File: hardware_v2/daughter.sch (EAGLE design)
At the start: 25 parts, among them K1 PIN20X2, U1 EEPROM24, U2 MCP2551-I/SN, U4 TPS27081A, X1 MABC48B2

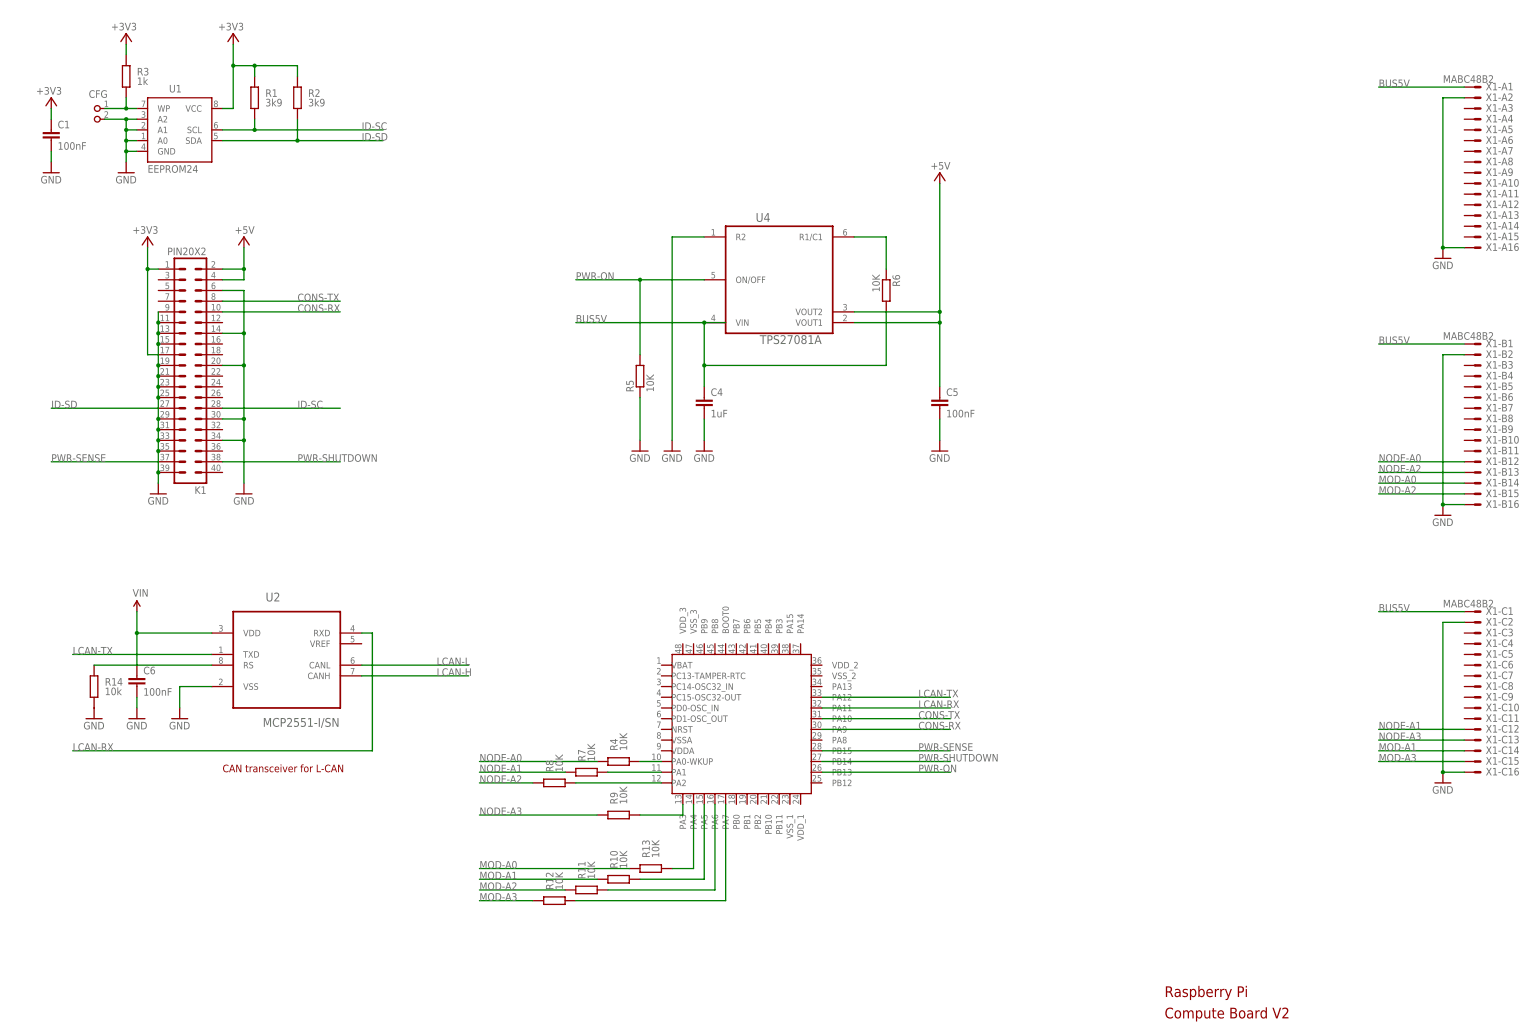
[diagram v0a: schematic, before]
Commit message: hardware_v2: build in STM32
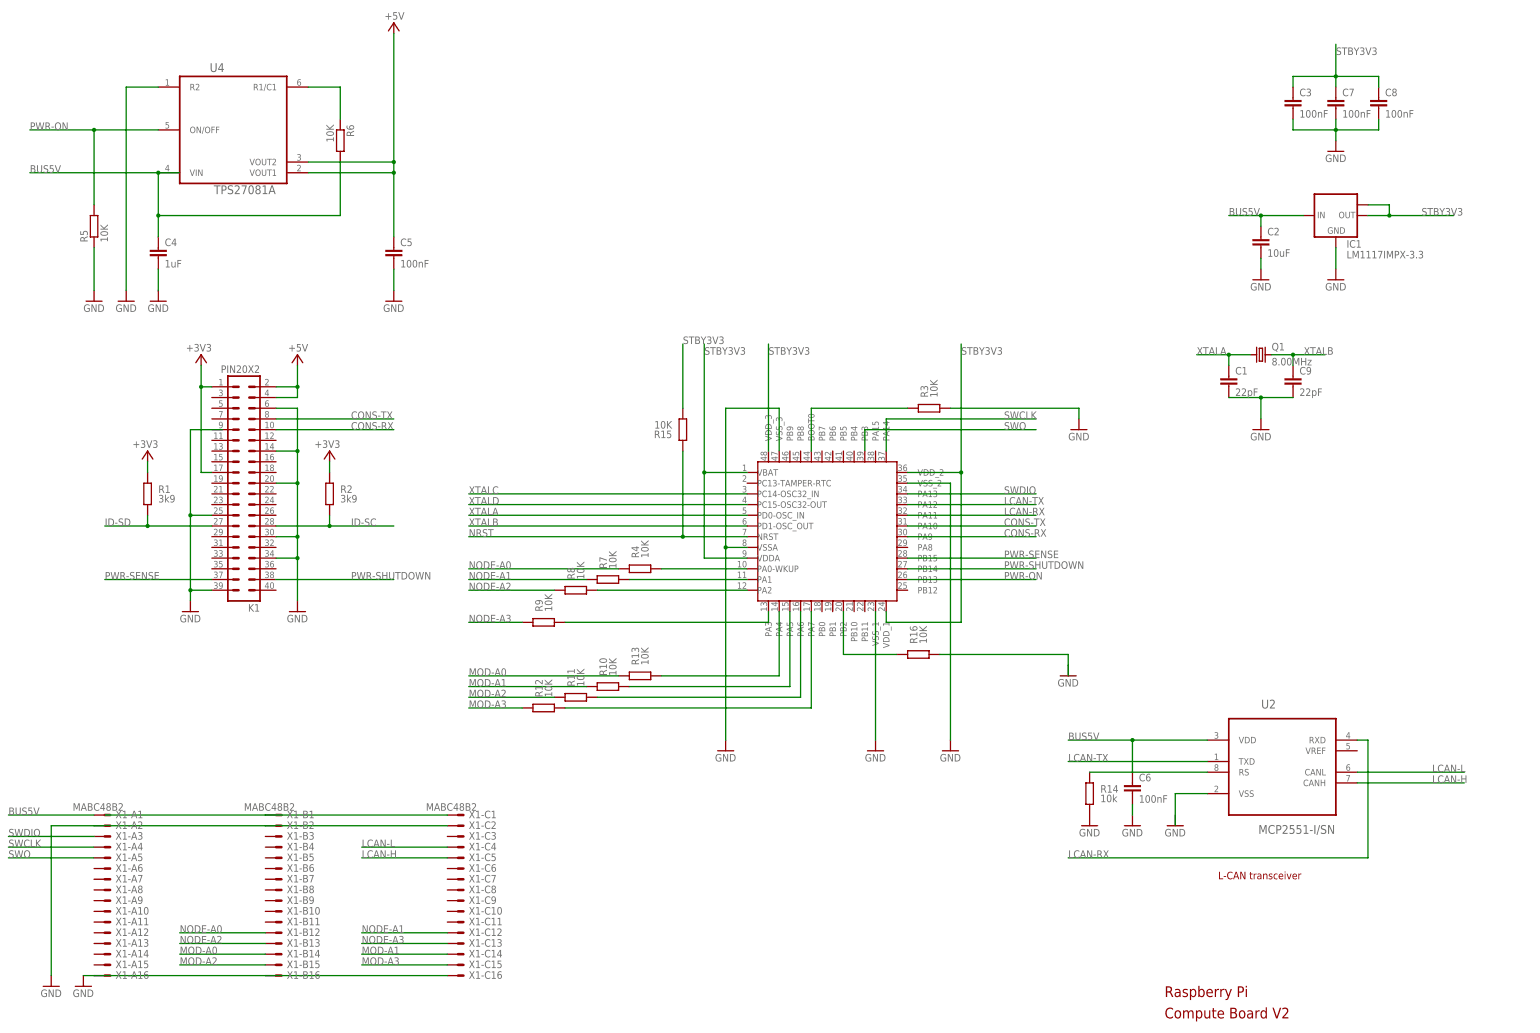
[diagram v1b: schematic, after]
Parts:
- removed CFG: (no value), FLYFISH:PIN2_100
- removed U1: EEPROM24, FLYFISH:EEPROM24
- added C2: 10uF, resistor:C-EUC0805K
- added C3, C7, C8: 100nF, resistor:C-EUC0805K
- added C9: 22pF, resistor:C-EUC1206
- added IC1: LM1117IMPX-3.3, lm1117:LM1117IMPX-3.3
- added Q1: 8.00MHz, crystal:CRYSTALSM49
- added R15, R16: 10K, resistor:R-EU_M0805
- C1: value 100nF -> 22pF; device resistor:C-EUC0805K -> resistor:C-EUC1206; DIELECTRIC X7R -> (none)
- R3: value 1k -> 10K
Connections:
- removed net VIN: C6.1, U2.VDD
- new net N$11: R16.2, U$1.PB2
- new net N$12: U2.VSS
- new net NRST: R15.2, U$1.NRST
- new net STBY3V3: C3.1, C7.1, C8.1, IC1.OUT, IC1.OUT1, R15.1, U$1.VBAT, U$1.VDDA, U$1.VDD_1, U$1.VDD_2, U$1.VDD_3
- new net SWCLK: U$1.PA14, X1-A4.S
- new net SWDIO: U$1.PA13, X1-A3.S
- new net SWO: U$1.PB3, X1-A5.S
- new net XTALA: C1.1, Q1.1, U$1.PD0-OSC_IN
- new net XTALB: C9.1, Q1.2, U$1.PD1-OSC_OUT
- new net XTALC: U$1.PC14-OSC32_IN
- new net XTALD: U$1.PC15-OSC32-OUT
- net +3V3: no longer C1.1, R3.2, U1.VCC
- net BUS5V: now also C2.1, C6.1, IC1.IN, U2.VDD
- net GND: now also C2.2, C3.2, C7.2, C8.2, C9.2, IC1.GND, R16.1, R3.1, U$1.VSSA, U$1.VSS_1, U$1.VSS_2, U$1.VSS_3; no longer CFG.2, K1.11, K1.13, K1.15, K1.19, K1.21, K1.23, K1.29, K1.31, K1.33, K1.35, K1.9, U1.A0, U1.A1, U1.A2, U1.GND
- net ID-SC: now also R2.1; no longer R1.1, U1.SCL
- net ID-SD: now also R1.1; no longer R2.1, U1.SDA
- net LCAN-H: now also X1-C5.S
- net LCAN-L: now also X1-C4.S
- net N$3: now also R3.2, U$1.BOOT0; no longer CFG.1, R3.1, U1.WP
- net N$4: no longer U2.VSS
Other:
- note added: "L-CAN transceiver"
- note removed: "CAN transceiver for L-CAN"
- moved on the sheet: C1, C4, C5, C6, K1, R1, R10, R11, R12, R13, R14, R2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
